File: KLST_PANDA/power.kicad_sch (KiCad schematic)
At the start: 9 parts, among them Q1 AO3401A, U1 AMS1117-3.3

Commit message: assigned footprints
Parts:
- NT1: footprint NetTie-2_SMD_Pad2.0mm -> NetTie:NetTie-2_SMD_Pad2.0mm
- U1: JLCPCB (none) -> C6186; JLCPCB Part # C6186 -> (none)
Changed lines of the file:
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@@
       (effects (font (size 1.27 1.27)) hide)
     )
-    (property "JLCPCB Part #" "C6186" (at 76.2 38.735 0)
+    (property "JLCPCB Part #" "" (at 76.2 38.735 0)
+      (effects (font (size 1.27 1.27)) hide)
+    )
+    (property "JLCPCB" "C6186" (at 76.2 38.735 0)
       (effects (font (size 1.27 1.27)) hide)
     )
@@
       (effects (font (size 1.27 1.27)) (justify left))
     )
-    (property "Footprint" "NetTie-2_SMD_Pad2.0mm" (at 92.075 30.48 0)
+    (property "Footprint" "NetTie:NetTie-2_SMD_Pad2.0mm" (at 92.075 30.48 0)
       (effects (font (size 1.27 1.27)) hide)
     )

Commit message: cleaned up footprint assignment
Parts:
- C1, C3: Extended Part - -> (none); MFR.Part # CL21A106KAYNNNE -> (none)
- C4: Extended Part - -> (none); MFR.Part # CL05A105KA5NQNC -> (none)
- C5: Extended Part - -> (none); MFR.Part # CL05B103KB5NNNC -> (none)
- L1: Extended Part - -> (none); MFR.Part # SDCL1005C39NJTDF -> (none)
- Q1: Extended Part - -> (none); MFR.Part # AO3401A -> (none)
- U1: Extended Part - -> (none); MFR.Part # AMS1117-3.3 -> (none)
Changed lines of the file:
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@@
-      (effects (font (size 1.27 1.27)) hide)
-    )
-    (property "MFR.Part #" "CL21A106KAYNNNE" (at 92.075 45.085 0)
-      (effects (font (size 1.27 1.27)) hide)
-    )
-    (property "LCSC Part #" "" (at 92.075 45.085 0)
-      (effects (font (size 1.27 1.27)) hide)
-    )
-    (property "Extended Part" "-" (at 92.075 45.085 0)
-      (effects (font (size 1.27 1.27)) hide)
-    )
-    (property "JLCPCB Part #" "" (at 92.075 45.085 0)
       (effects (font (size 1.27 1.27)) hide)
     )
@@
     )
     (property "Datasheet" "~" (at 53.34 38.735 0)
-      (effects (font (size 1.27 1.27)) hide)
-    )
-    (property "JLCPCB Part #" "" (at 53.34 38.735 90)
       (effects (font (size 1.27 1.27)) hide)
     )
@@
       (effects (font (size 1.27 1.27)) hide)
     )
-    (property "MFR.Part #" "CL05B103KB5NNNC" (at 135.89 34.29 0)
-      (effects (font (size 1.27 1.27)) hide)
-    )
-    (property "LCSC Part #" "" (at 135.89 34.29 0)
-      (effects (font (size 1.27 1.27)) hide)
-    )
-    (property "Extended Part" "-" (at 135.89 34.29 0)
-      (effects (font (size 1.27 1.27)) hide)
-    )
-    (property "JLCPCB Part #" "" (at 135.89 34.29 0)
-      (effects (font (size 1.27 1.27)) hide)
-    )
     (property "JLCPCB" "C1710" (at 135.89 34.29 0)
       (effects (font (size 1.27 1.27)) hide)
@@
       (effects (font (size 1.27 1.27)) hide)
     )
-    (property "MFR.Part #" "CL05A105KA5NQNC" (at 125.73 34.29 0)
-      (effects (font (size 1.27 1.27)) hide)
-    )
-    (property "LCSC Part #" "" (at 125.73 34.29 0)
-      (effects (font (size 1.27 1.27)) hide)
-    )
-    (property "Extended Part" "-" (at 125.73 34.29 0)
-      (effects (font (size 1.27 1.27)) hide)
-    )
-    (property "JLCPCB Part #" "" (at 125.73 34.29 0)
-      (effects (font (size 1.27 1.27)) hide)
-    )
     (property "JLCPCB" "C28323" (at 125.73 34.29 0)
       (effects (font (size 1.27 1.27)) hide)
@@
       (effects (font (size 1.27 1.27)) hide)
     )
-    (property "MFR.Part #" "SDCL1005C39NJTDF" (at 120.65 30.48 90)
-      (effects (font (size 1.27 1.27)) hide)
-    )
-    (property "LCSC Part #" "" (at 120.65 30.48 90)
-      (effects (font (size 1.27 1.27)) hide)
-    )
-    (property "Extended Part" "-" (at 120.65 30.48 0)
-      (effects (font (size 1.27 1.27)) hide)
-    )
-    (property "JLCPCB Part #" "" (at 120.65 30.48 0)
-      (effects (font (size 1.27 1.27)) hide)
-    )
     (property "JLCPCB" "C26443" (at 120.65 30.48 0)
       (effects (font (size 1.27 1.27)) hide)
@@
       (effects (font (size 1.27 1.27)) hide)
     )
-    (property "MFR.Part #" "CL21A106KAYNNNE" (at 62.23 45.085 0)
-      (effects (font (size 1.27 1.27)) hide)
-    )
-    (property "LCSC Part #" "" (at 62.23 45.085 0)
-      (effects (font (size 1.27 1.27)) hide)
-    )
-    (property "Extended Part" "-" (at 62.23 45.085 0)
-      (effects (font (size 1.27 1.27)) hide)
-    )
-    (property "JLCPCB Part #" "" (at 62.23 45.085 0)
-      (effects (font (size 1.27 1.27)) hide)
-    )
     (property "Description" "25V" (at 62.23 45.085 0)
       (effects (font (size 1.27 1.27)) hide)
@@
       (effects (font (size 1.27 1.27)) (justify left) hide)
     )
-    (property "MFR.Part #" "AO3401A" (at 38.1 41.275 90)
-      (effects (font (size 1.27 1.27)) hide)
-    )
-    (property "LCSC Part #" "" (at 38.1 41.275 90)
-      (effects (font (size 1.27 1.27)) hide)
-    )
-    (property "Extended Part" "-" (at 38.1 41.275 0)
-      (effects (font (size 1.27 1.27)) hide)
-    )
-    (property "JLCPCB Part #" "" (at 38.1 41.275 0)
-      (effects (font (size 1.27 1.27)) hide)
-    )
     (property "JLCPCB" "C15127" (at 38.1 41.275 0)
       (effects (font (size 1.27 1.27)) hide)
@@
       (effects (font (size 1.27 1.27)) hide)
     )
-    (property "MFR.Part #" "AMS1117-3.3" (at 76.2 38.735 0)
-      (effects (font (size 1.27 1.27)) hide)
-    )
-    (property "Extended Part" "-" (at 76.2 38.735 0)
-      (effects (font (size 1.27 1.27)) hide)
-    )
-    (property "JLCPCB Part #" "" (at 76.2 38.735 0)
-      (effects (font (size 1.27 1.27)) hide)
-    )

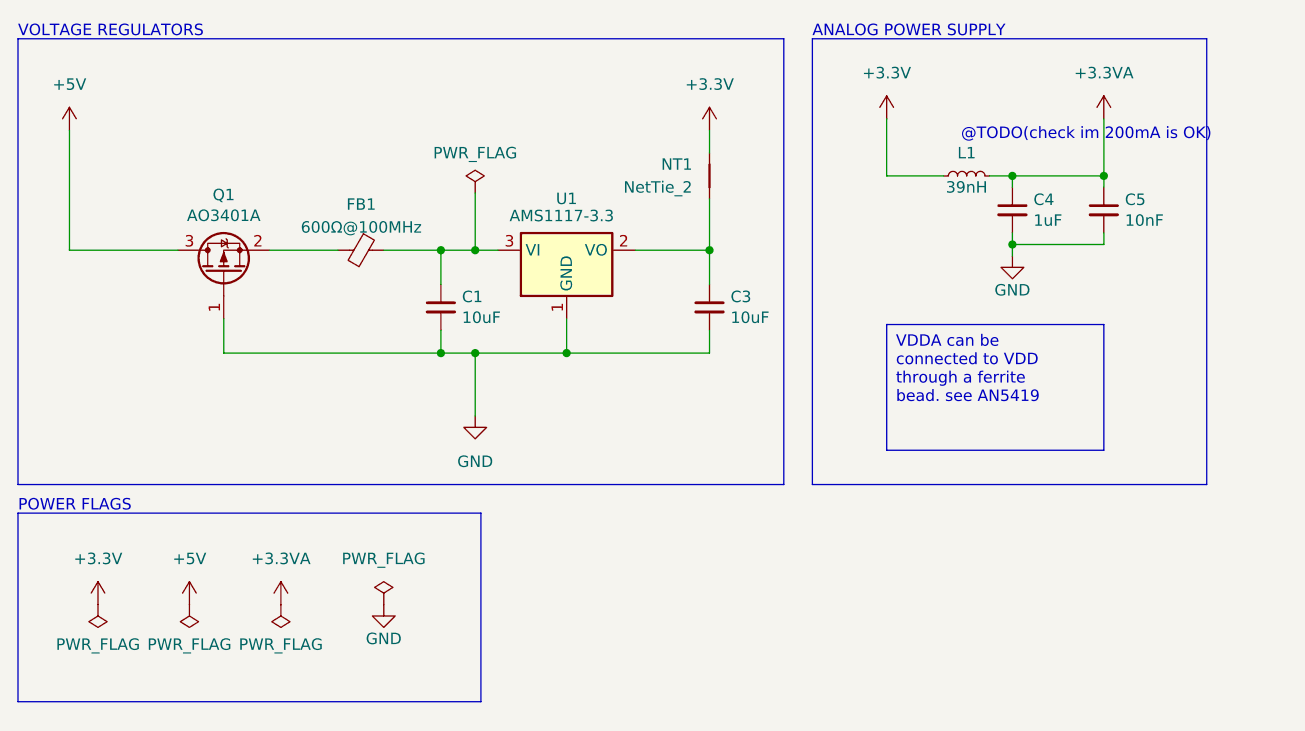
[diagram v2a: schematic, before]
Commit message: distributed modules
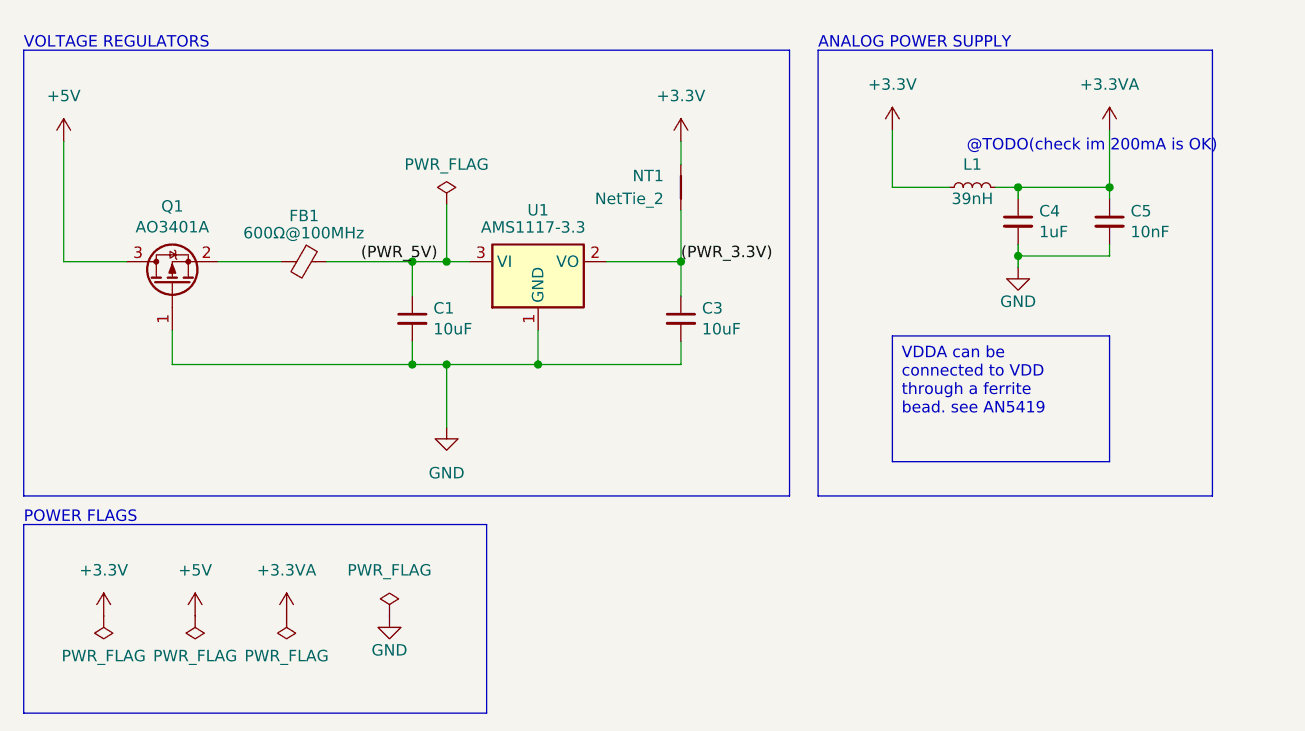
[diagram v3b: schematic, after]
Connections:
- net (PWR_3.3V): now reaches C3.1, NT1.2, U1.2 (VO)
- net (PWR_5V): now reaches C1.1, FB1.1, U1.3 (VI)
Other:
- moved on the sheet: C1, C3, C4, C5, FB1, L1, NT1, Q1, U1
